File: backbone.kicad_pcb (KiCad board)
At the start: 2 copper layers, 55.6 x 95.6 mm, 6 parts, among them J1 Communication, J2 Borta, J3 Sensor, J4 Power, J5 CAM_1, J6 CAM_2

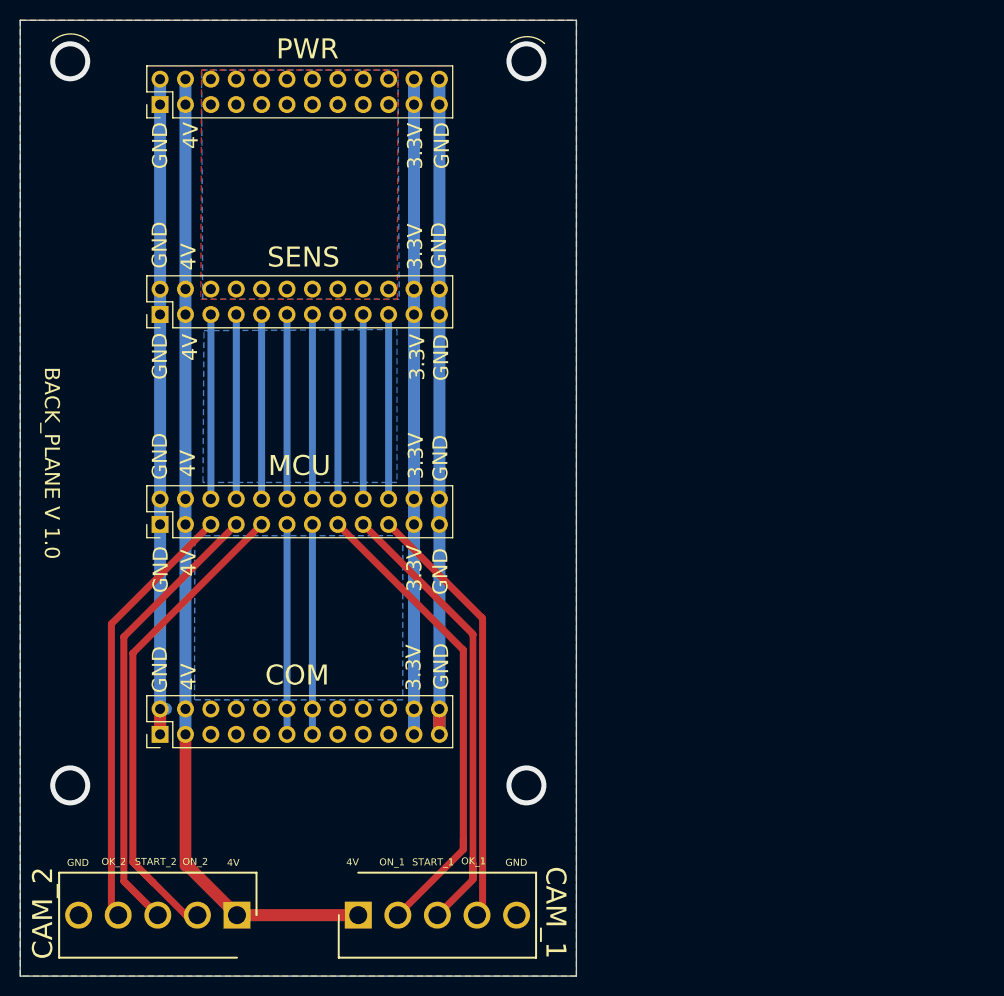
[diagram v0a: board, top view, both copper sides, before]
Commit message: 0.1v
Ridiculess backbone
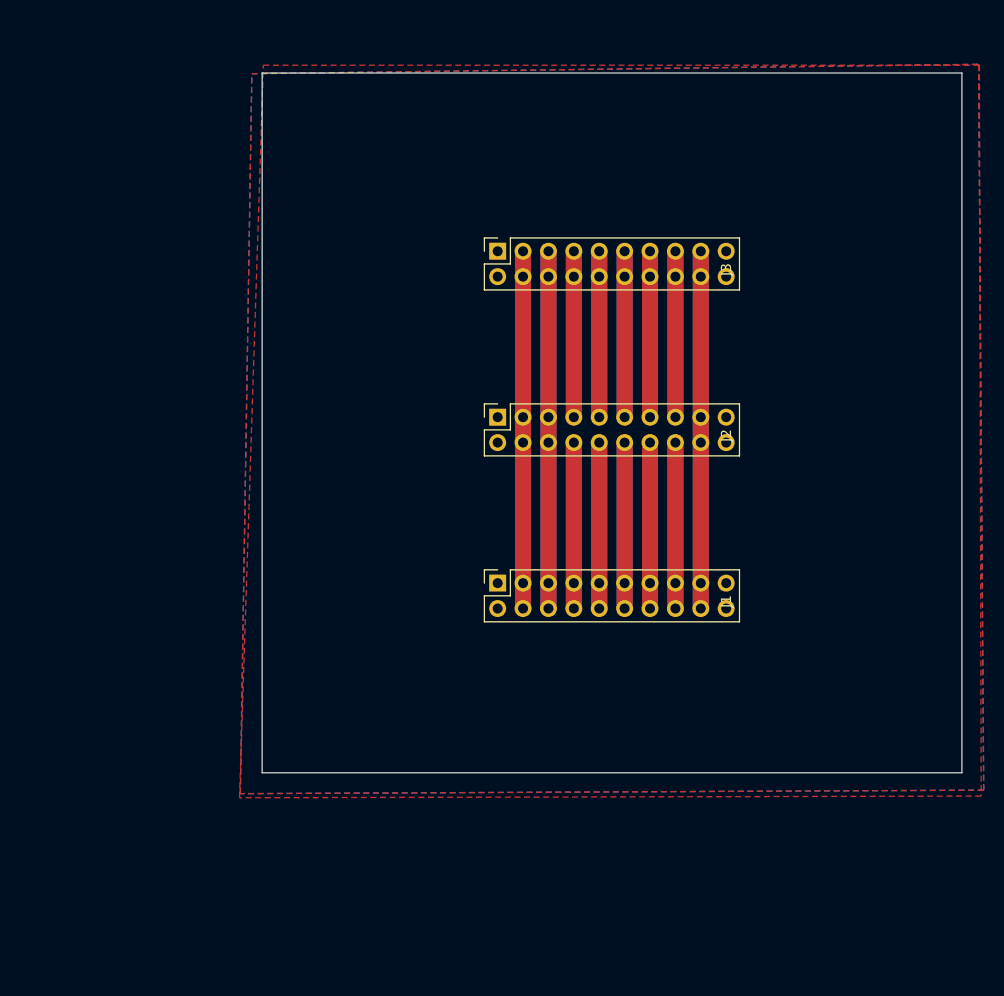
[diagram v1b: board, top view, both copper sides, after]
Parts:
- removed J4: Power, LOCAL:PinHeader_2x12_P2.54mm_Vertical
- removed J5: CAM_1, LOCAL:HDRV5W114P0X396_1X5_1974X850X1070P
- removed J6: CAM_2, LOCAL:HDRV5W114P0X396_1X5_1974X850X1070P
- J1, J2: footprint LOCAL:PinHeader_2x12_P2.54mm_Vertical -> Connector_PinSocket_2.54mm:PinSocket_2x10_P2.54mm_Vertical
- J3: value Sensor -> Power; footprint LOCAL:PinHeader_2x12_P2.54mm_Vertical -> Connector_PinSocket_2.54mm:PinSocket_2x10_P2.54mm_Vertical
- moved J1 37.0 mm to (165.1, 100.4)
- moved J2 35.4 mm to (165.1, 83.8)
- moved J3 34.4 mm to (165.1, 67.2)
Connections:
- J1 pad 1: (no net) -> GND
- J1 pad 10: (no net) -> MCU_RX_COM_TX
- J1 pad 11: (no net) -> MCU_TX_COM_RX
- J1 pad 12: (no net) -> MCU_TX_COM_RX
- J1 pad 13: (no net) -> NC1
- J1 pad 14: (no net) -> NC1
- J1 pad 15: (no net) -> NC2
- J1 pad 16: (no net) -> NC2
- J1 pad 17: (no net) -> 3.3V
- J1 pad 18: (no net) -> 3.3V
- J1 pad 19: (no net) -> GND
- J1 pad 2: (no net) -> GND
- J1 pad 20: (no net) -> GND
- J1 pad 3: (no net) -> 4V
- J1 pad 4: (no net) -> 4V
- J1 pad 5: (no net) -> NC
- J1 pad 6: (no net) -> NC
- J1 pad 7: (no net) -> NC0
- J1 pad 8: (no net) -> NC0
- J1 pad 9: (no net) -> MCU_RX_COM_TX
- J2 pad 1: (no net) -> GND
- J2 pad 10: (no net) -> MCU_RX_COM_TX
- J2 pad 11: (no net) -> ADC_4V
- J2 pad 12: (no net) -> MCU_TX_COM_RX
- J2 pad 13: (no net) -> ROPE_CUT
- J2 pad 14: (no net) -> NC1
- J2 pad 15: (no net) -> BUZZER
- J2 pad 16: (no net) -> NC2
- J2 pad 17: (no net) -> 3.3V
- J2 pad 18: (no net) -> 3.3V
- J2 pad 19: (no net) -> GND
- J2 pad 2: (no net) -> GND
- J2 pad 20: (no net) -> GND
- J2 pad 3: (no net) -> 4V
- J2 pad 4: (no net) -> 4V
- J2 pad 5: (no net) -> NC
- J2 pad 6: (no net) -> NC
- J2 pad 7: (no net) -> ADC_VBAT
- J2 pad 8: (no net) -> NC0
- J2 pad 9: (no net) -> ADC_3.3V
- J3 pad 1: (no net) -> GND
- J3 pad 10: (no net) -> ADC_3.3V
- J3 pad 11: (no net) -> ADC_4V
- J3 pad 12: (no net) -> ADC_4V
- J3 pad 13: (no net) -> ROPE_CUT
- J3 pad 14: (no net) -> ROPE_CUT
- J3 pad 15: (no net) -> BUZZER
- J3 pad 16: (no net) -> BUZZER
- J3 pad 17: (no net) -> 3.3V
- J3 pad 18: (no net) -> 3.3V
- J3 pad 19: (no net) -> GND
- J3 pad 2: (no net) -> GND
- J3 pad 20: (no net) -> GND
- J3 pad 3: (no net) -> 4V
- J3 pad 4: (no net) -> 4V
- J3 pad 5: (no net) -> NC
- J3 pad 6: (no net) -> NC
- J3 pad 7: (no net) -> ADC_VBAT
- J3 pad 8: (no net) -> ADC_VBAT
- J3 pad 9: (no net) -> ADC_3.3V
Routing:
- net (no net): track 771.6 -> 0.00 mm, vias 4 -> 0
- net NC: track 0.00 -> 71.5 mm
- net 4V: track 0.00 -> 71.5 mm
- net 3.3V: track 0.00 -> 71.5 mm
- net ROPE_CUT: track 0.00 -> 33.2 mm
- net NC2: track 0.00 -> 33.2 mm
- net NC1: track 0.00 -> 33.2 mm
- net NC0: track 0.00 -> 33.2 mm
- net MCU_TX_COM_RX: track 0.00 -> 33.2 mm
- net MCU_RX_COM_TX: track 0.00 -> 33.2 mm
- net BUZZER: track 0.00 -> 33.2 mm
- net ADC_VBAT: track 0.00 -> 33.2 mm
- net ADC_4V: track 0.00 -> 33.2 mm
- net ADC_3.3V: track 0.00 -> 33.2 mm
- added copper zone on B.Cu, net GND
- added copper zone on F.Cu, net GND
- removed copper zone on B.Cu, net (none)
- removed copper zone on F.Cu, net (none)
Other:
- board size 55.6 x 95.6 mm -> 70 x 70 mm
- board text removed: "3.3V"
- board text removed: "4V"
- board text removed: "BACK_PLANE V 1.0"
- board text removed: "CAM_1"
- board text removed: "CAM_2"
- board text removed: "COM"
- board text removed: "GND"
- board text removed: "MCU"
- board text removed: "OK_1"
- board text removed: "OK_2"
- board text removed: "ON_1"
- board text removed: "ON_2"
- board text removed: "PWR"
- board text removed: "SENS"
- board text removed: "START_1"
- board text removed: "START_2"
